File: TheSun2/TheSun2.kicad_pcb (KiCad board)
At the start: 2 copper layers, 65 x 30 mm, 37 parts, among them J5 Conn_02x20_Odd_Even, Q1 IRLR7843, Q2 IRLR7843, Q3 IRLR7843, Q4 IRLR7843, U1 2N7002H, U2 2N7002H, U3 2N7002H, U4 2N7002H, U5 2N7002H, U6 2N7002H, U7 2N7002H, U8 2N7002H

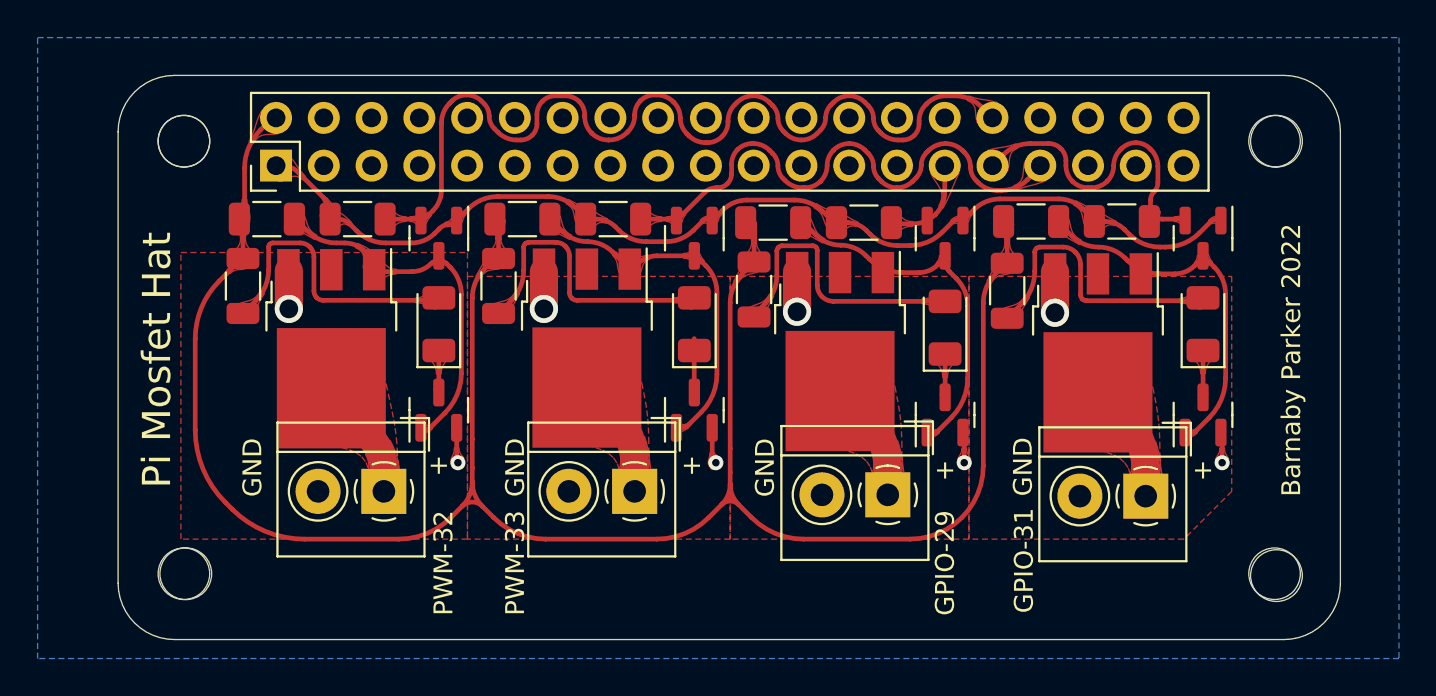
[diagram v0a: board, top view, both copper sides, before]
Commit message: Added first draft for pi mosfethat
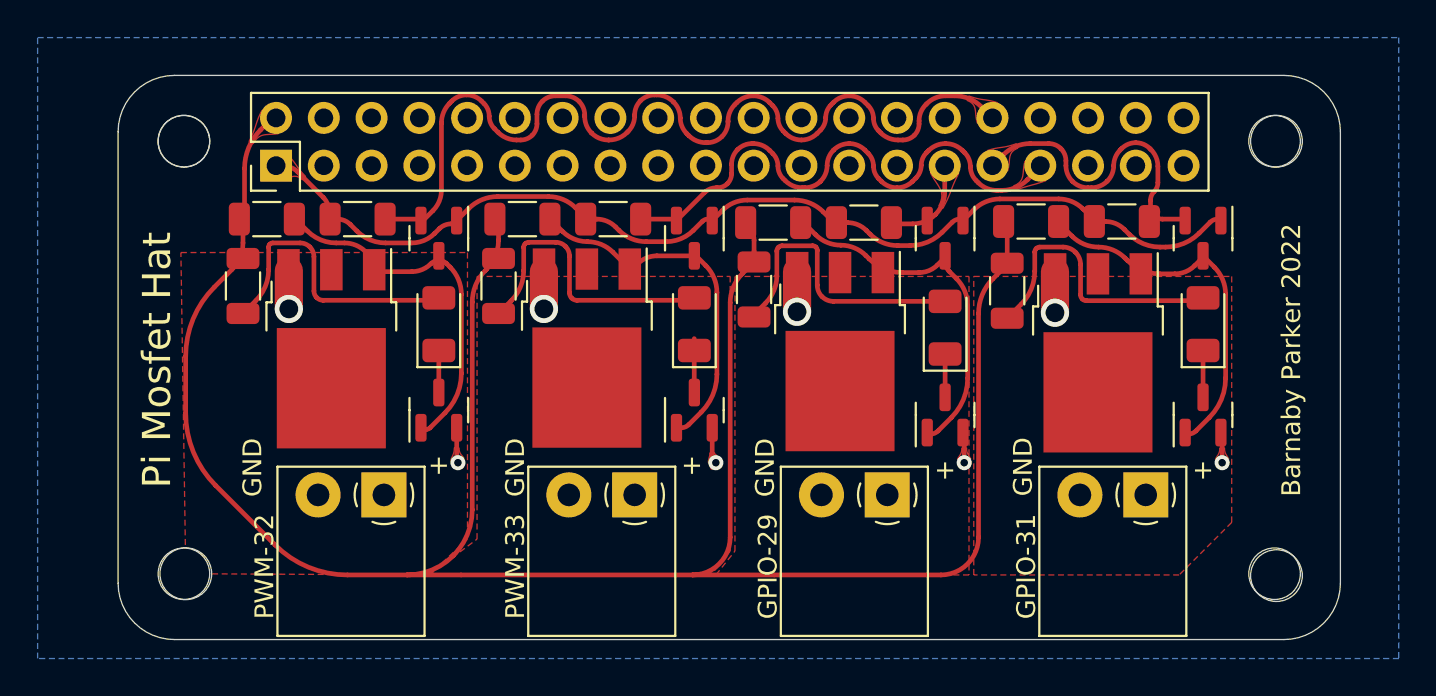
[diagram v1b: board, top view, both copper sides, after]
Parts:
- added G***: LOGO, LOGO, B.Cu at (82.5, 62.6)
- GPIO-29, GPIO-31, PWM-32, PWM-33: footprint TerminalBlock_4Ucon:TerminalBlock_4Ucon_1x02_P3.50mm_Horizontal -> BSP-Custom:TerminalBlock_4Ucon_1x02_P3.50mm_Horizontal
- moved PWM-32 0.19 mm to (64.1, 71.3)
- moved PWM-33 0.19 mm to (77.5, 71.3)
- moved GPIO-31 0.07 mm to (104.6, 71.3)
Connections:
- PWM-32 pad 1: Net-(Q1-Pad2) -> Net-(J1-Pad1)
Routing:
- net 5v: track 115.7 -> 123.9 mm
- net Net-(J3-Pad1): track 6.46 -> 0.00 mm
- net Net-(J4-Pad1): track 6.46 -> 0.00 mm
- net Net-(J2-Pad1): track 6.40 -> 0.00 mm
- net Net-(J1-Pad1): track 6.16 -> 0.00 mm
